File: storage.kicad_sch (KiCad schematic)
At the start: 0 parts

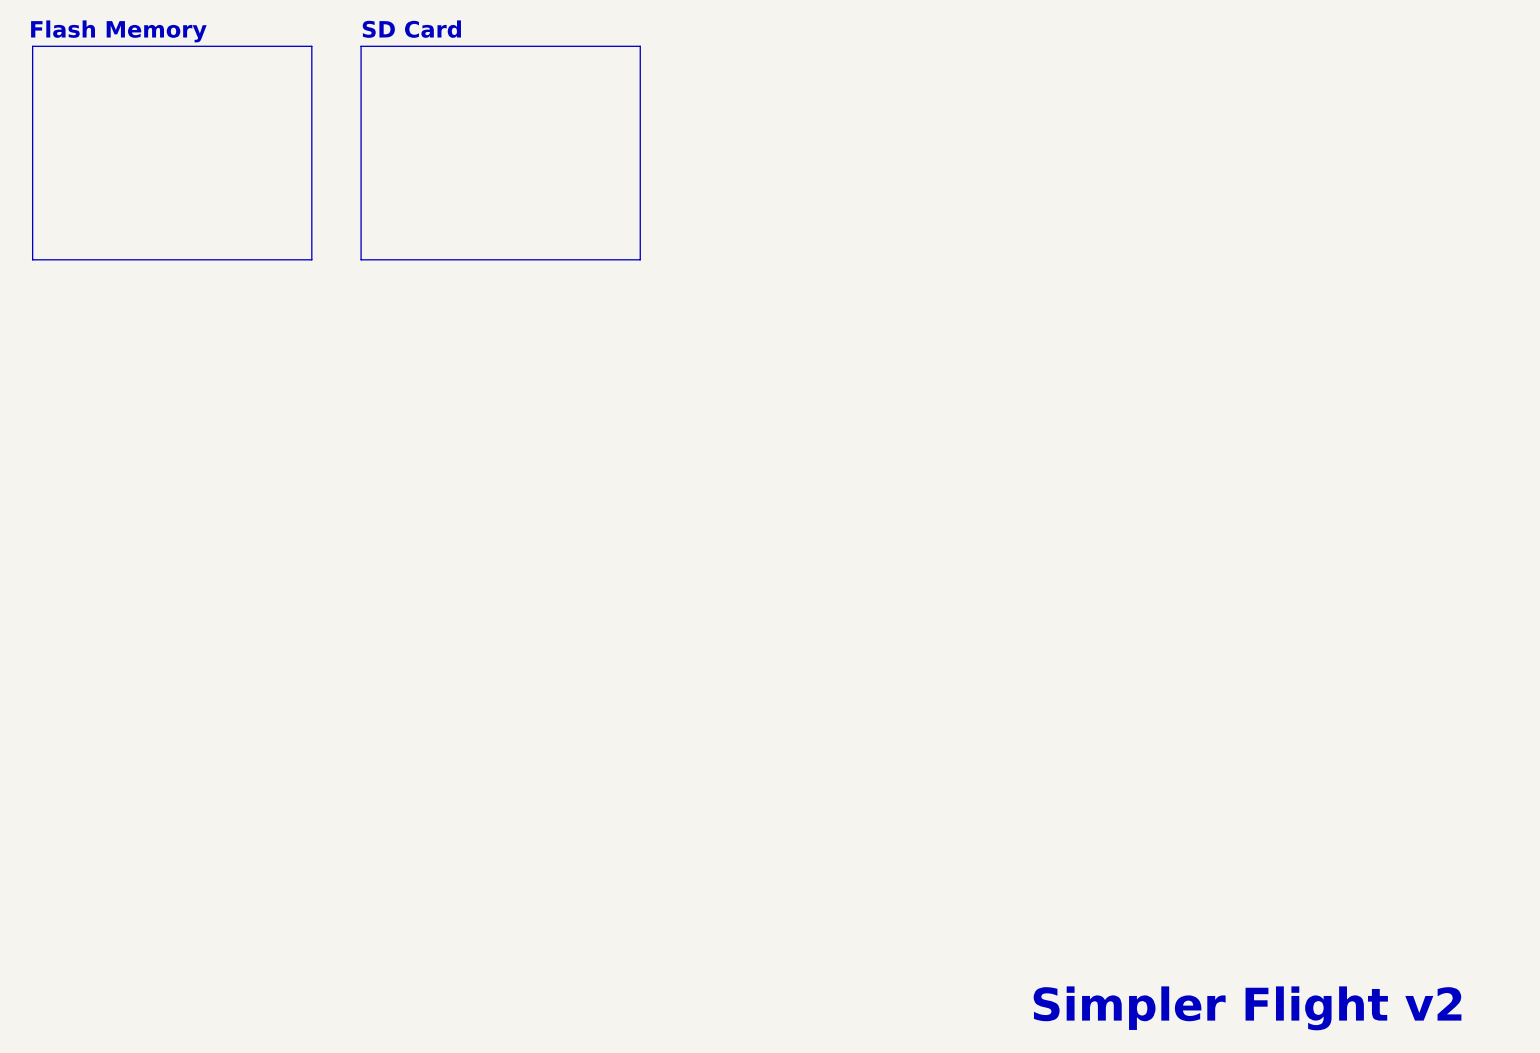
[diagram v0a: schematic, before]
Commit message: Initiliase main components
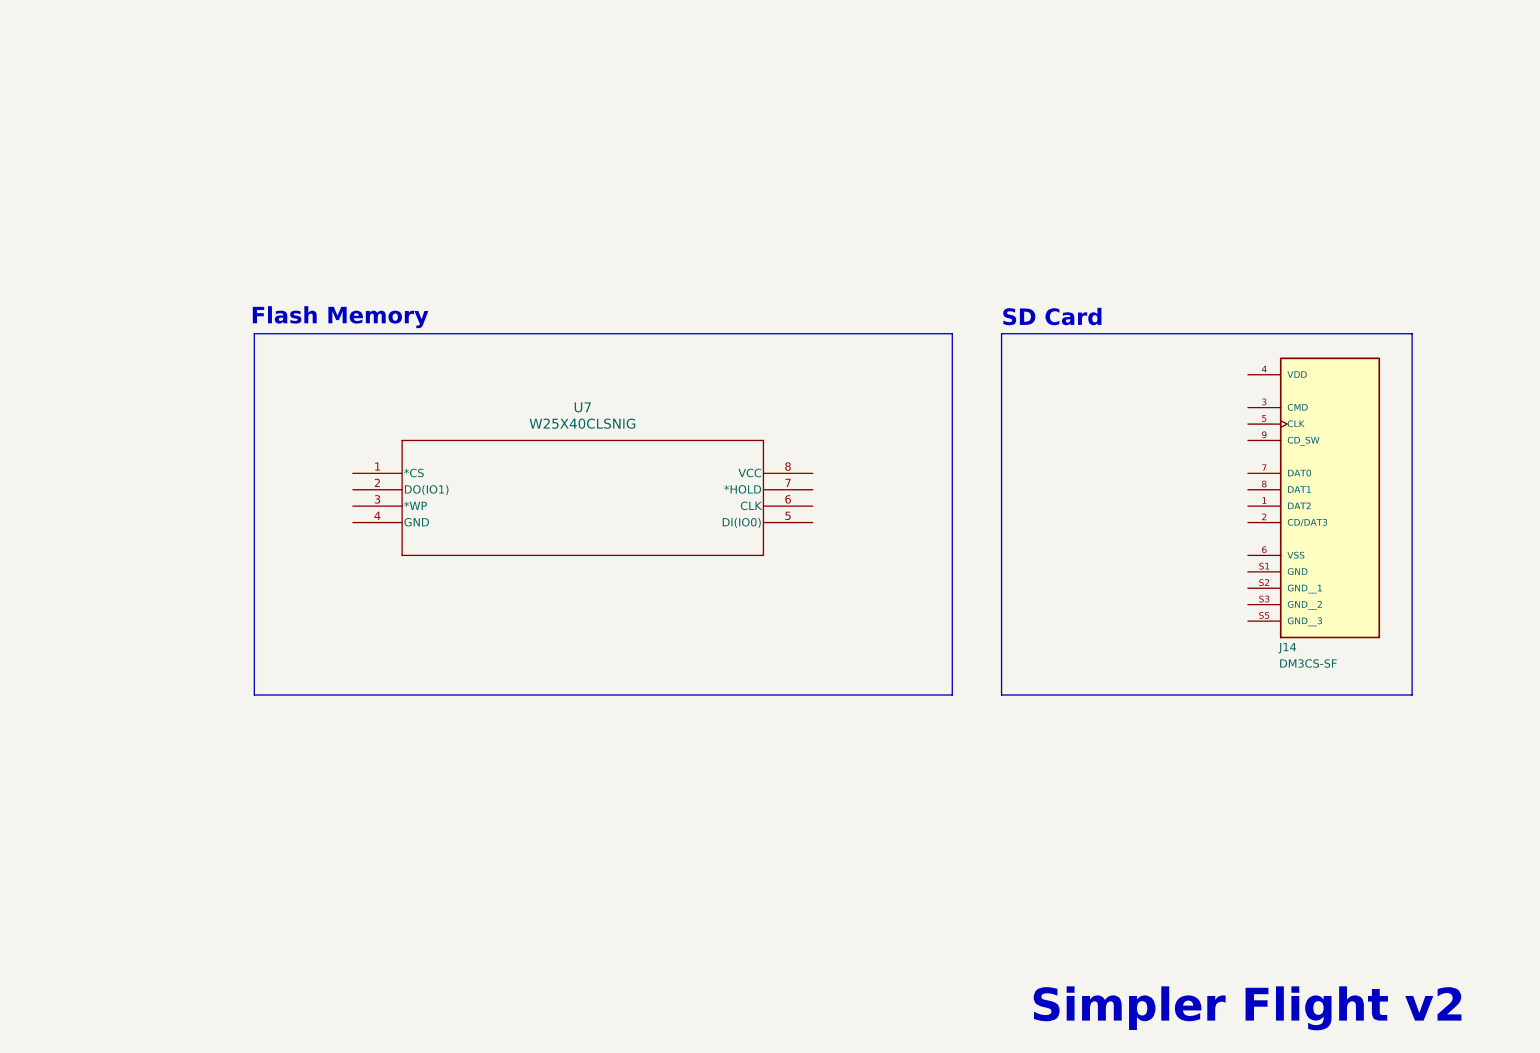
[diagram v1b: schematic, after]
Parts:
- added J14: DM3CS-SF, DM3CS_SF:HRS_DM3CS-SF, symbol DM3CS-SF:DM3CS-SF
- added U7: W25X40CLSNIG, W25X40CLSNIG:WIN_SN-8_WIN, symbol W25X40CLSNIG:W25X40CLSNIG
